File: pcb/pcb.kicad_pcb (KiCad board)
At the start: 2 copper layers, 75.2 x 62.6 mm, 39 parts, among them J1 Conn_01x06, U1 ATmega328P-AU, U2 SRV05-4

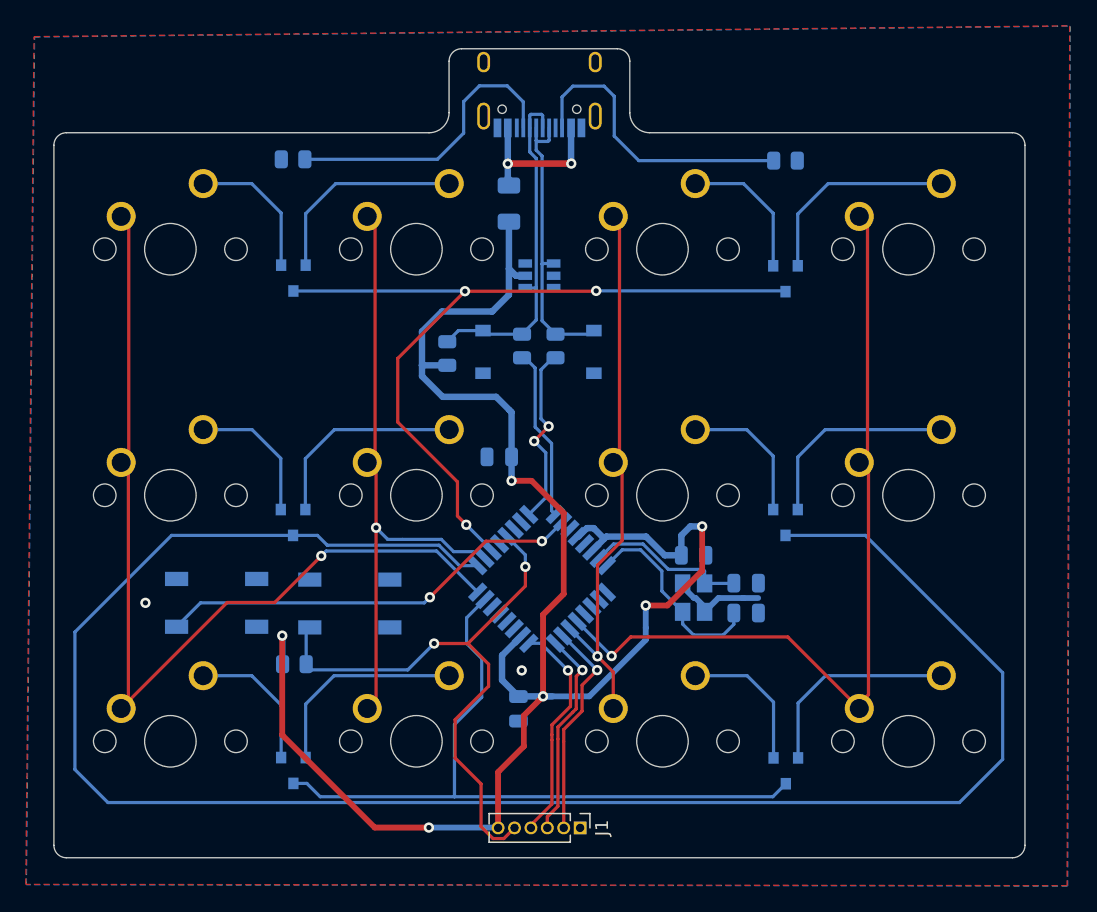
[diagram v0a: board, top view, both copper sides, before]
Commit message: add readme and fabrication files
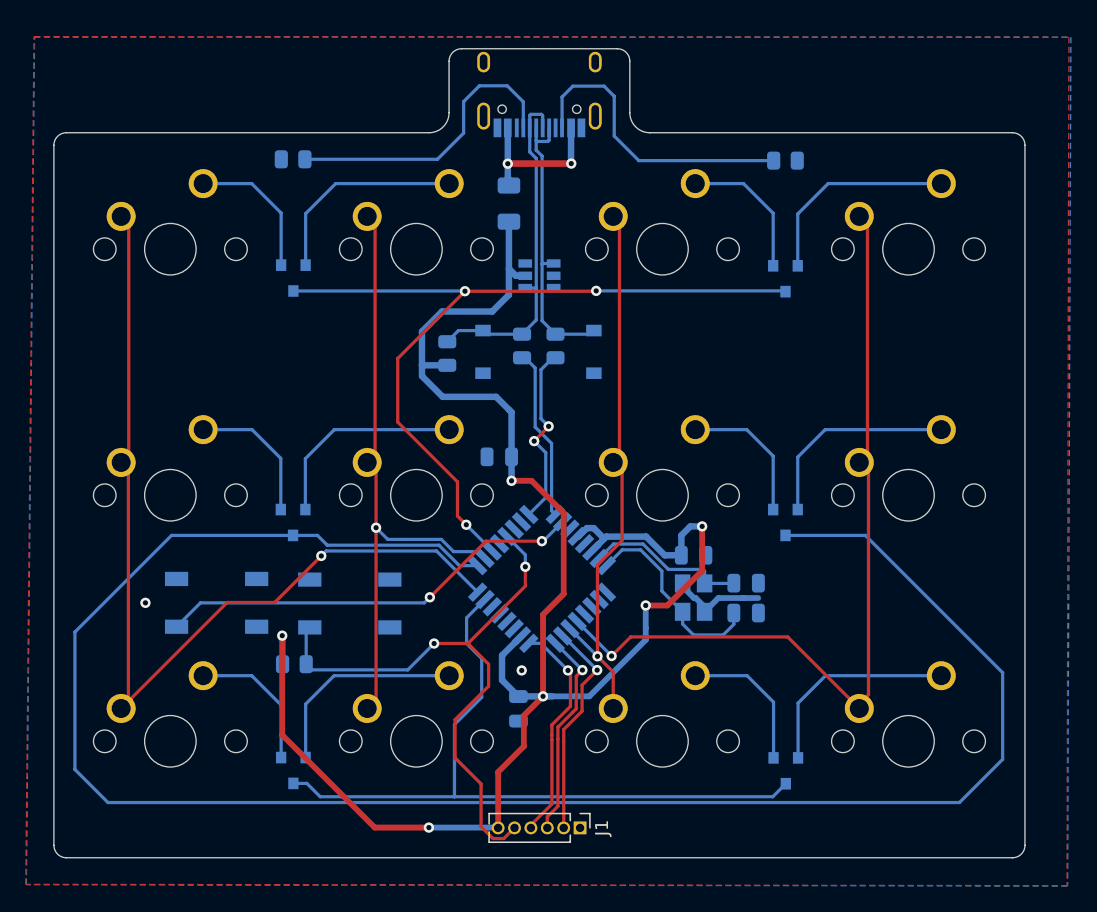
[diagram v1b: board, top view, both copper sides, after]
